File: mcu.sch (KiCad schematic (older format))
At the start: 18 parts, among them J501 JTAG, J502 Serial / Bootloader, SW501 EVQQ2, SW502 EVQQ2, U501 STM32F405RGTx, Y501 8MHz

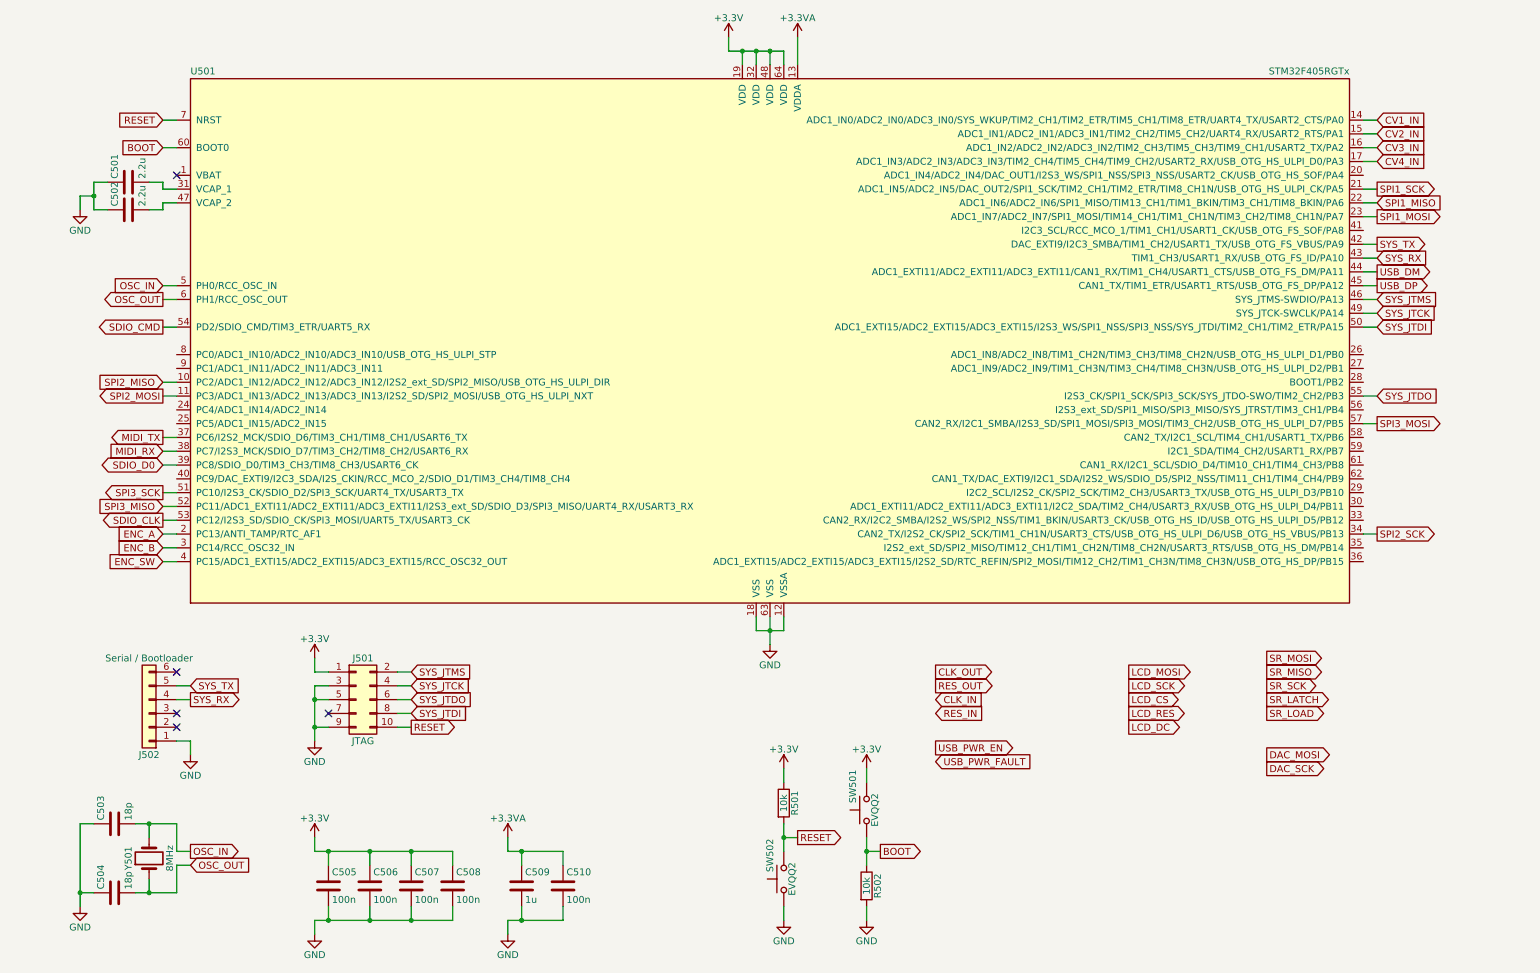
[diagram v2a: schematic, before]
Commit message: more work on layout
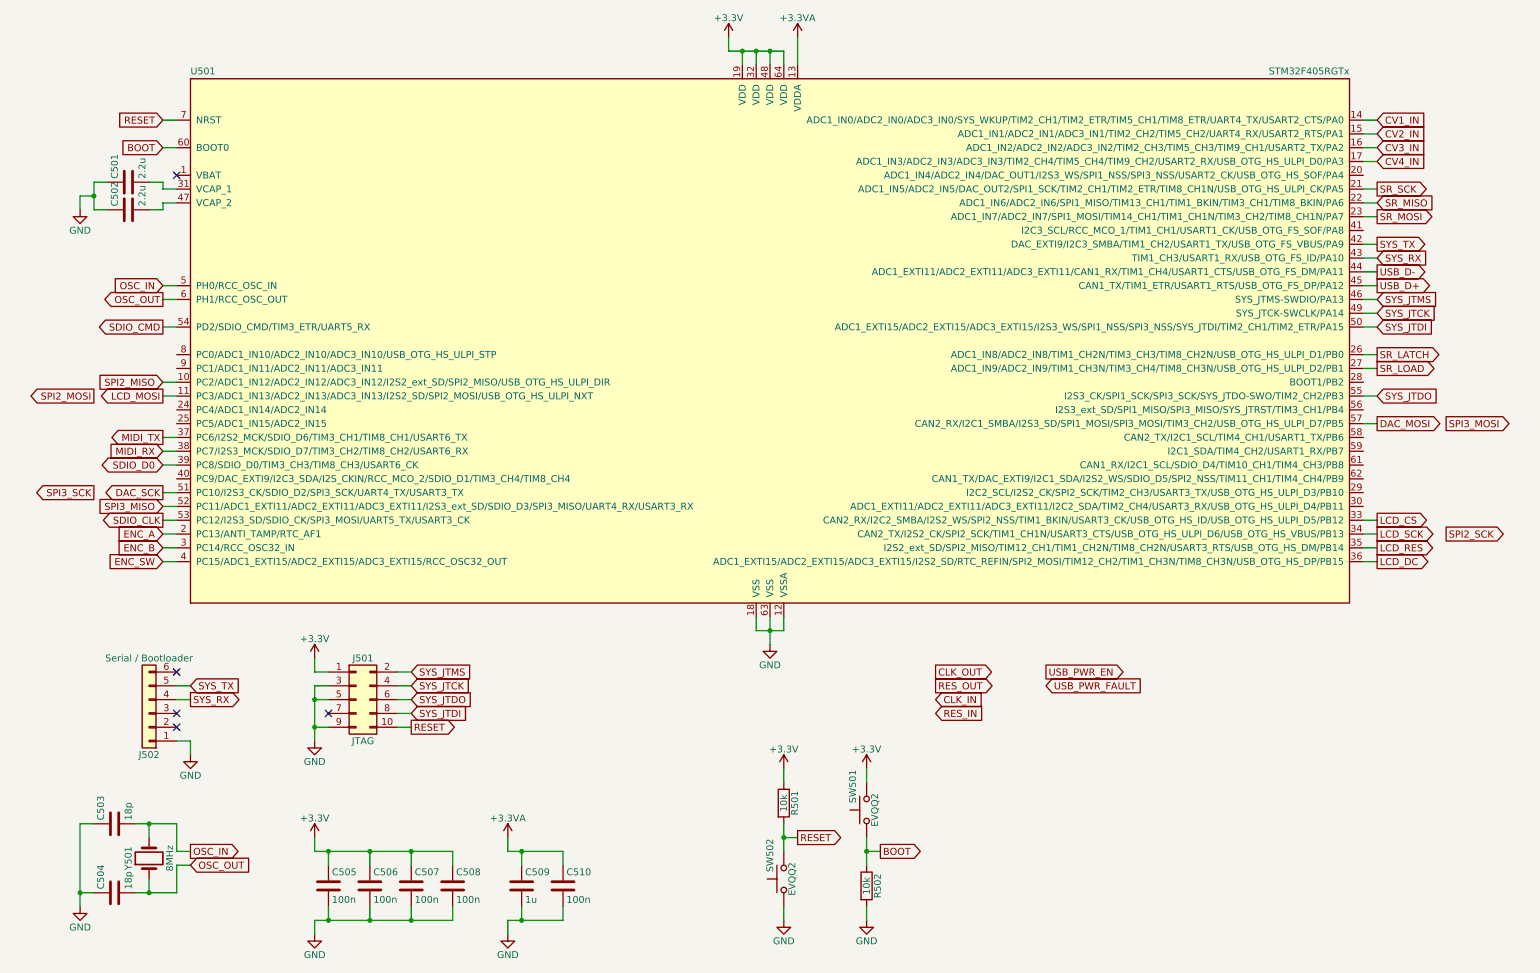
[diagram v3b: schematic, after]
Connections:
- net SPI1_MISO is gone; now on net SR_MISO: U501.22 (ADC1_IN6/ADC2_IN6/SPI1_MISO/TIM13_CH1/TIM1_BKIN/TIM3_CH1/TIM8_BKIN/PA6)
- net SPI1_MOSI is gone; now on net SR_MOSI: U501.23 (ADC1_IN7/ADC2_IN7/SPI1_MOSI/TIM14_CH1/TIM1_CH1N/TIM3_CH2/TIM8_CH1N/PA7)
- net SPI1_SCK is gone; now on net SR_SCK: U501.21 (ADC1_IN5/ADC2_IN5/DAC_OUT2/SPI1_SCK/TIM2_CH1/TIM2_ETR/TIM8_CH1N/USB_OTG_HS_ULPI_CK/PA5)
- net DAC_MOSI: now also U501.57 (CAN2_RX/I2C1_SMBA/I2S3_SD/SPI1_MOSI/SPI3_MOSI/TIM3_CH2/USB_OTG_HS_ULPI_D7/PB5)
- net DAC_SCK: now also U501.51 (PC10/I2S3_CK/SDIO_D2/SPI3_SCK/UART4_TX/USART3_TX)
- net LCD_CS: now also U501.33 (CAN2_RX/I2C2_SMBA/I2S2_WS/SPI2_NSS/TIM1_BKIN/USART3_CK/USB_OTG_HS_ID/USB_OTG_HS_ULPI_D5/PB12)
- net LCD_DC: now also U501.36 (ADC1_EXTI15/ADC2_EXTI15/ADC3_EXTI15/I2S2_SD/RTC_REFIN/SPI2_MOSI/TIM12_CH2/TIM1_CH3N/TIM8_CH3N/USB_OTG_HS_DP/PB15)
- net LCD_MOSI: now also U501.11 (PC3/ADC1_IN13/ADC2_IN13/ADC3_IN13/I2S2_SD/SPI2_MOSI/USB_OTG_HS_ULPI_NXT)
- net LCD_RES: now also U501.35 (I2S2_ext_SD/SPI2_MISO/TIM12_CH1/TIM1_CH2N/TIM8_CH2N/USART3_RTS/USB_OTG_HS_DM/PB14)
- net LCD_SCK: now also U501.34 (CAN2_TX/I2S2_CK/SPI2_SCK/TIM1_CH1N/USART3_CTS/USB_OTG_HS_ULPI_D6/USB_OTG_HS_VBUS/PB13)
- net SPI2_MOSI: no longer U501.11 (PC3/ADC1_IN13/ADC2_IN13/ADC3_IN13/I2S2_SD/SPI2_MOSI/USB_OTG_HS_ULPI_NXT)
- net SPI2_SCK: no longer U501.34 (CAN2_TX/I2S2_CK/SPI2_SCK/TIM1_CH1N/USART3_CTS/USB_OTG_HS_ULPI_D6/USB_OTG_HS_VBUS/PB13)
- net SPI3_MOSI: no longer U501.57 (CAN2_RX/I2C1_SMBA/I2S3_SD/SPI1_MOSI/SPI3_MOSI/TIM3_CH2/USB_OTG_HS_ULPI_D7/PB5)
- net SPI3_SCK: no longer U501.51 (PC10/I2S3_CK/SDIO_D2/SPI3_SCK/UART4_TX/USART3_TX)
- net SR_LATCH: now also U501.26 (ADC1_IN8/ADC2_IN8/TIM1_CH2N/TIM3_CH3/TIM8_CH2N/USB_OTG_HS_ULPI_D1/PB0)
- net SR_LOAD: now also U501.27 (ADC1_IN9/ADC2_IN9/TIM1_CH3N/TIM3_CH4/TIM8_CH3N/USB_OTG_HS_ULPI_D2/PB1)
- net USB_DM renamed USB_D-
- net USB_DP renamed USB_D+
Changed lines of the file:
@@
 Text GLabel 1400 4000 0    51   Input ~ 0
 MIDI_RX
-Text GLabel 8400 5600 2    51   Output ~ 0
+Text GLabel 1400 3600 0    51   Output ~ 0
 LCD_MOSI
-Text GLabel 8400 5700 2    51   Output ~ 0
+Text GLabel 10200 4600 2    51   Output ~ 0
 LCD_SCK
-Text GLabel 8400 5800 2    51   Output ~ 0
+Text GLabel 10200 4500 2    51   Output ~ 0
 LCD_CS
-Text GLabel 8400 5900 2    51   Output ~ 0
+Text GLabel 10200 4700 2    51   Output ~ 0
 LCD_RES
-Text GLabel 8400 6000 2    51   Output ~ 0
+Text GLabel 10200 4800 2    51   Output ~ 0
 LCD_DC
 Text GLabel 1400 4600 0    51   Input ~ 0
@@
 Text GLabel 1400 4800 0    51   Input ~ 0
 ENC_SW
-Text GLabel 10200 2100 2    51   Output ~ 0
-SPI1_SCK
-Text GLabel 10200 2200 2    51   Input ~ 0
-SPI1_MISO
-Text GLabel 10200 2300 2    51   Output ~ 0
-SPI1_MOSI
 Text GLabel 1400 3500 0    51   Input ~ 0
 SPI2_MISO
-Text GLabel 1400 3600 0    51   Output ~ 0
+Text GLabel 900  3600 0    51   Output ~ 0
 SPI2_MOSI
-Text GLabel 10200 4600 2    51   Output ~ 0
+Text GLabel 10700 4600 2    51   Output ~ 0
 SPI2_SCK
-Text GLabel 10200 3800 2    51   Output ~ 0
+Text GLabel 10700 3800 2    51   Output ~ 0
 SPI3_MOSI
-Text GLabel 1400 4300 0    51   Output ~ 0
+Text GLabel 900  4300 0    51   Output ~ 0
 SPI3_SCK
 Text GLabel 1400 4400 0    51   Input ~ 0
@@
 Text GLabel 7000 5900 2    51   Input ~ 0
 RES_IN
-Text GLabel 9400 5500 2    51   Output ~ 0
+Text GLabel 10200 2300 2    51   Output ~ 0
 SR_MOSI
-Text GLabel 9400 5600 2    51   Output ~ 0
+Text GLabel 10200 2200 2    51   Input ~ 0
 SR_MISO
-Text GLabel 9400 5700 2    51   Output ~ 0
+Text GLabel 10200 2100 2    51   Output ~ 0
 SR_SCK
-Text GLabel 9400 5800 2    51   Output ~ 0
+Text GLabel 10200 3300 2    51   Output ~ 0
 SR_LATCH
-Text GLabel 9400 5900 2    51   Output ~ 0
+Text GLabel 10200 3400 2    51   Output ~ 0
 SR_LOAD
-Text GLabel 9400 6200 2    51   Output ~ 0
+Text GLabel 10200 3800 2    51   Output ~ 0
 DAC_MOSI
-Text GLabel 9400 6300 2    51   Output ~ 0
+Text GLabel 1400 4300 0    51   Output ~ 0
 DAC_SCK
-Text GLabel 7000 6150 2    51   Output ~ 0
+Text GLabel 7800 5600 2    51   Output ~ 0
 USB_PWR_EN
-Text GLabel 7000 6250 2    51   Input ~ 0
+Text GLabel 7800 5700 2    51   Input ~ 0
 USB_PWR_FAULT
 Text GLabel 10200 2700 2    51   Output ~ 0
-USB_DM
+USB_D-
 Text GLabel 10200 2800 2    51   Output ~ 0
-USB_DP
+USB_D+
 Wire Wire Line
 	1500 6100 1600 6100
@@
 NoConn ~ 2600 5900
 NoConn ~ 1500 2000
+Wire Wire Line
+	10100 3300 10200 3300
+Wire Wire Line
+	10100 3400 10200 3400
+Wire Wire Line
+	10100 4500 10200 4500
+Wire Wire Line
+	10100 4700 10200 4700
+Wire Wire Line
+	10100 4800 10200 4800
 $EndSCHEMATC
